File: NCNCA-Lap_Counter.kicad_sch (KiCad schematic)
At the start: 3 parts

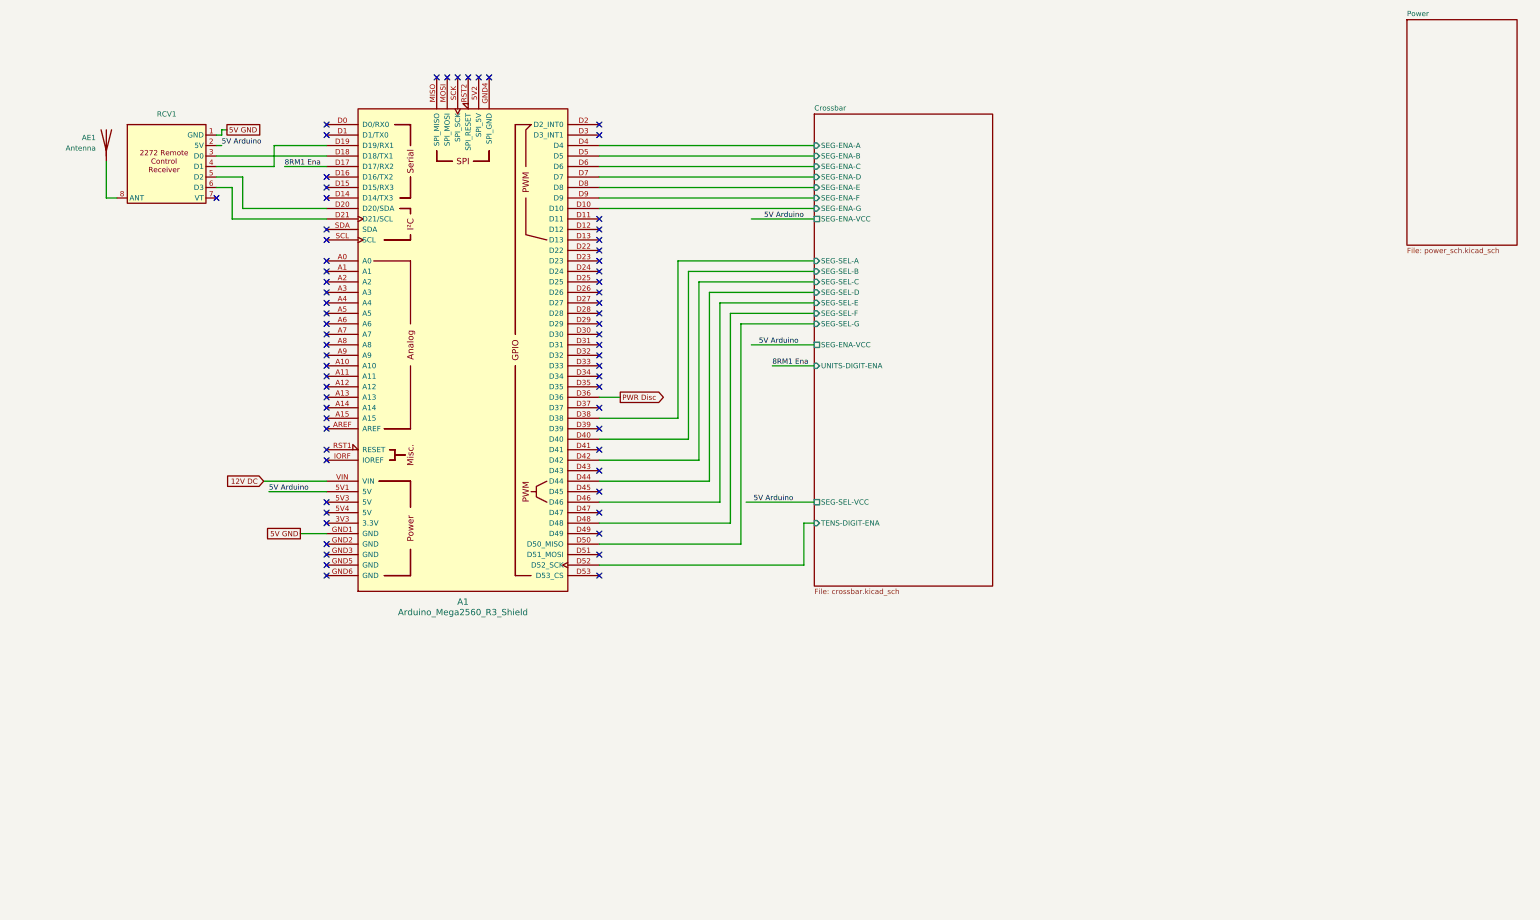
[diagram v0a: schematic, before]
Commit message: Misc clean up
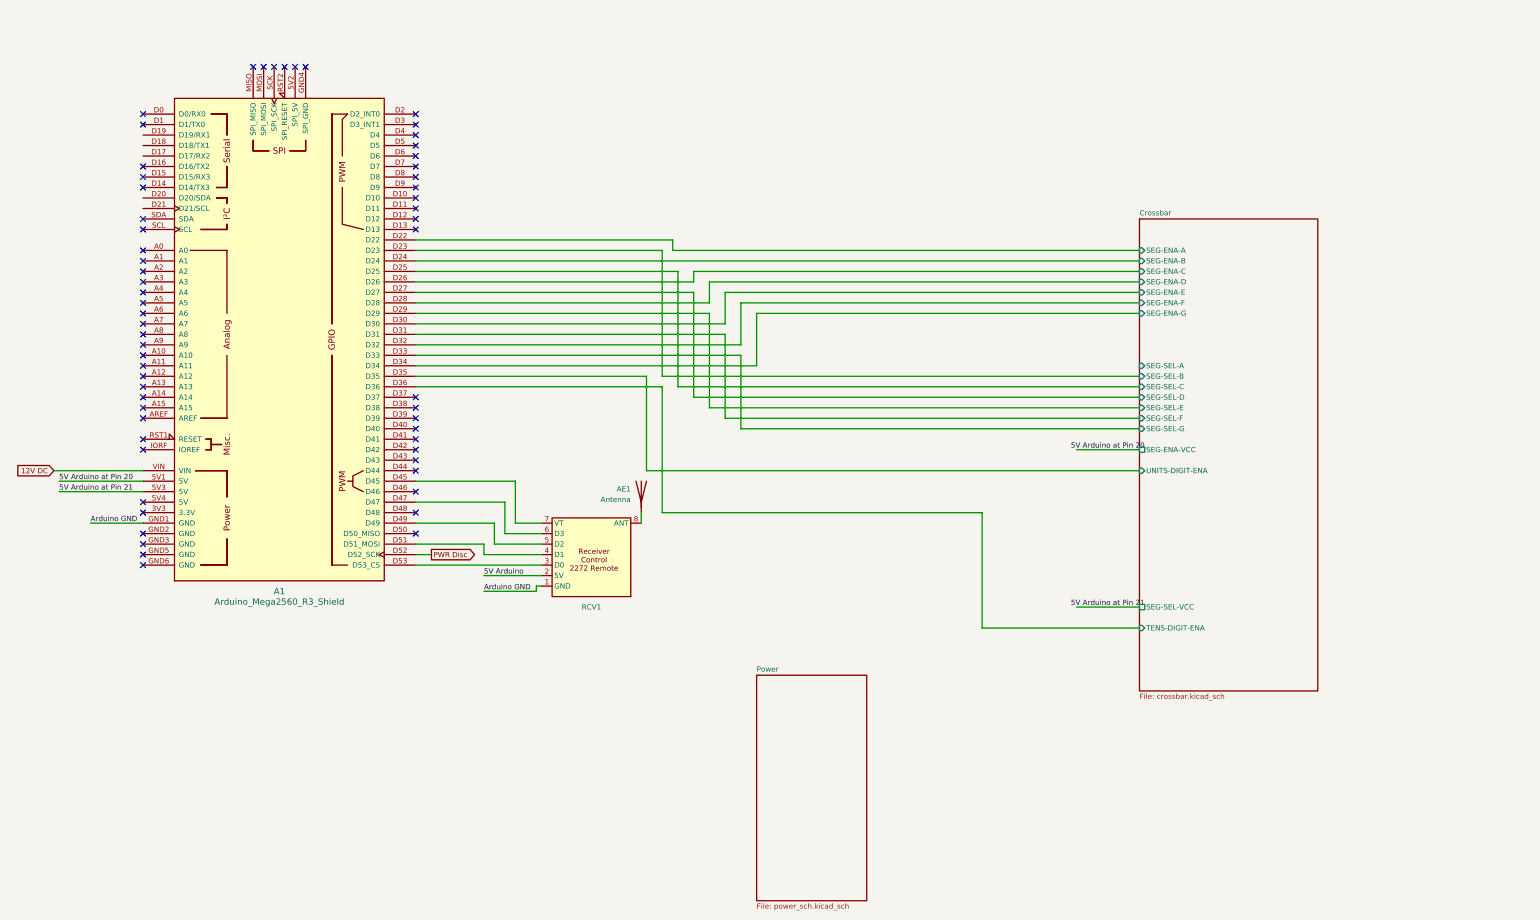
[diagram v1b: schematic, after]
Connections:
- net 5V Arduino: no longer A1.5V1 (5V)
- net Crossbar/SEG-ENA-A: now also A1.D22; no longer A1.D4
- net Crossbar/SEG-ENA-B: now also A1.D24; no longer A1.D5
- net Crossbar/SEG-ENA-C: now also A1.D26; no longer A1.D6
- net Crossbar/SEG-ENA-D: now also A1.D28; no longer A1.D7
- net Crossbar/SEG-ENA-E: now also A1.D30; no longer A1.D8
- net Crossbar/SEG-ENA-F: now also A1.D32; no longer A1.D9
- net Crossbar/SEG-ENA-G: now also A1.D34; no longer A1.D10
- net Crossbar/SEG-SEL-A: no longer A1.D38
- net Crossbar/SEG-SEL-B: now also A1.D23; no longer A1.D40
- net Crossbar/SEG-SEL-C: now also A1.D25; no longer A1.D42
- net Crossbar/SEG-SEL-D: now also A1.D27; no longer A1.D44
- net Crossbar/SEG-SEL-E: now also A1.D29; no longer A1.D46
- net Crossbar/SEG-SEL-F: now also A1.D31; no longer A1.D48
- net Crossbar/SEG-SEL-G: now also A1.D33; no longer A1.D50 (D50_MISO)
- net Crossbar/TENS-DIGIT-ENA: now also A1.D36; no longer A1.D52 (D52_SCK)
- net PWR Disc: now also A1.D52 (D52_SCK); no longer A1.D36
- net at RCV1.3 (D0): now also A1.D53 (D53_CS); no longer A1.D18 (D18/TX1)
- net at RCV1.4 (D1): now also A1.D51 (D51_MOSI); no longer A1.D19 (D19/RX1)
- net at RCV1.5 (D2): now also A1.D49; no longer A1.D20 (D20/SDA)
- net at RCV1.6 (D3): now also A1.D47; no longer A1.D21 (D21/SCL)
- net at RCV1.7 (VT): now also A1.D45
- net 5V Arduino at Pin 21: now reaches A1.5V3 (5V)
- net Crossbar/UNITS-DIGIT-ENA: now reaches A1.D35
- net 5V GND renamed Arduino GND
- net 8RM1 Ena: no longer names the net of A1.D17 (D17/RX2)
- new net 5V Arduino at Pin 20: A1.5V1 (5V)
- no-connect marks 68 -> 61
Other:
- moved on the sheet: A1, AE1, RCV1

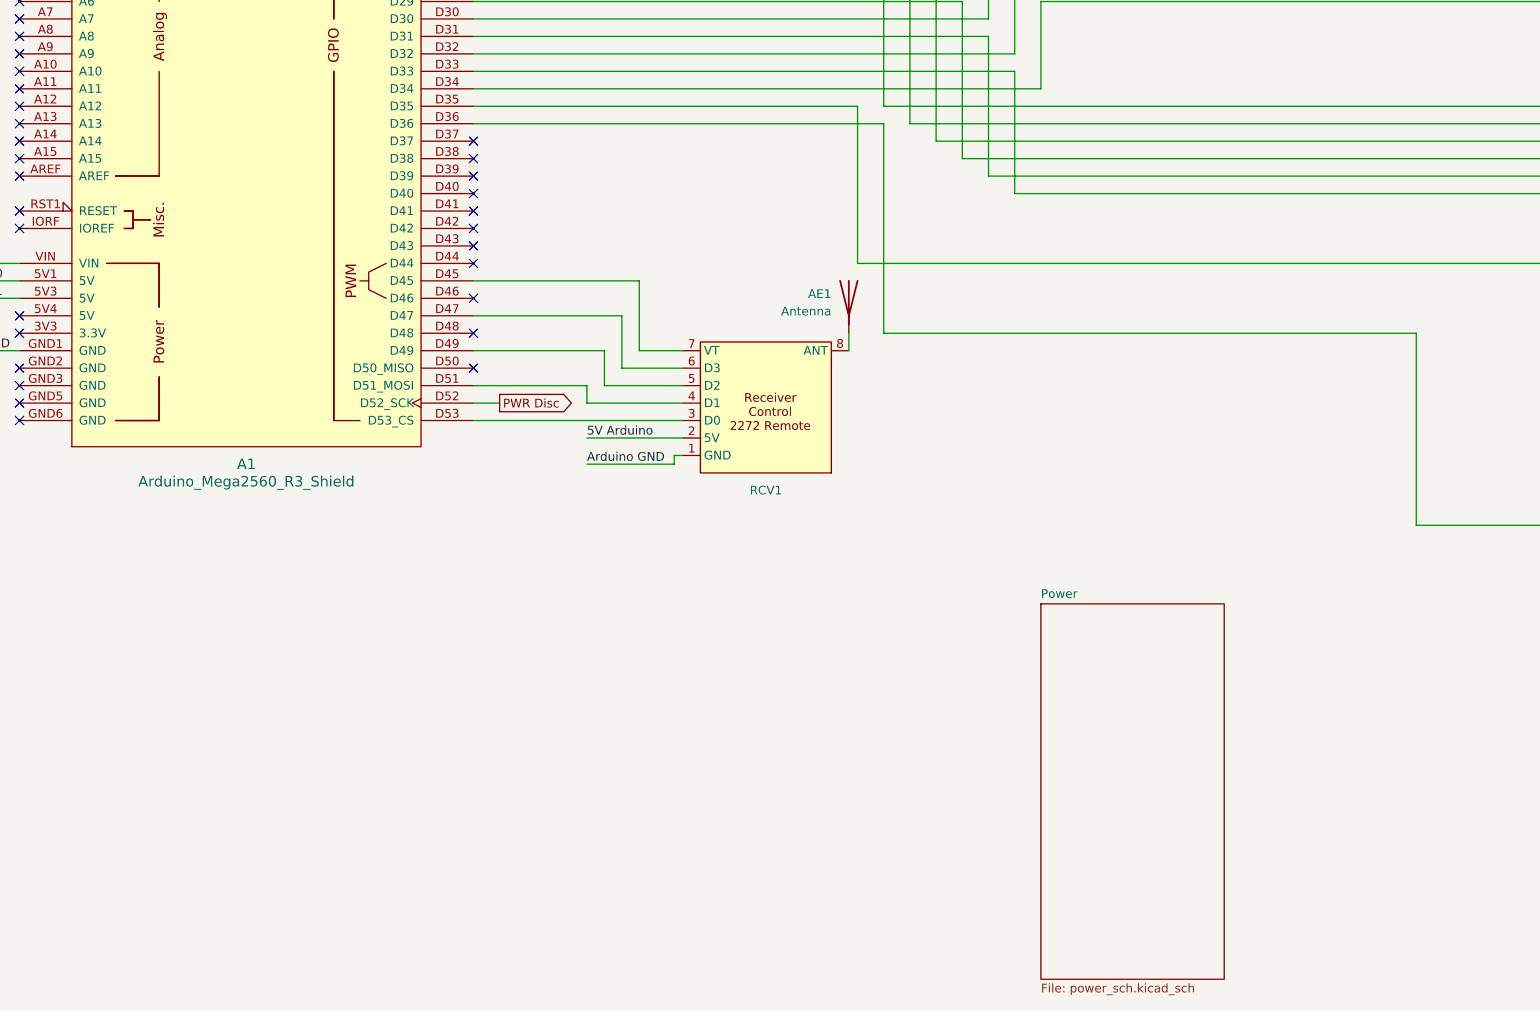
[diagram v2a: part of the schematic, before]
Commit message: Update documen
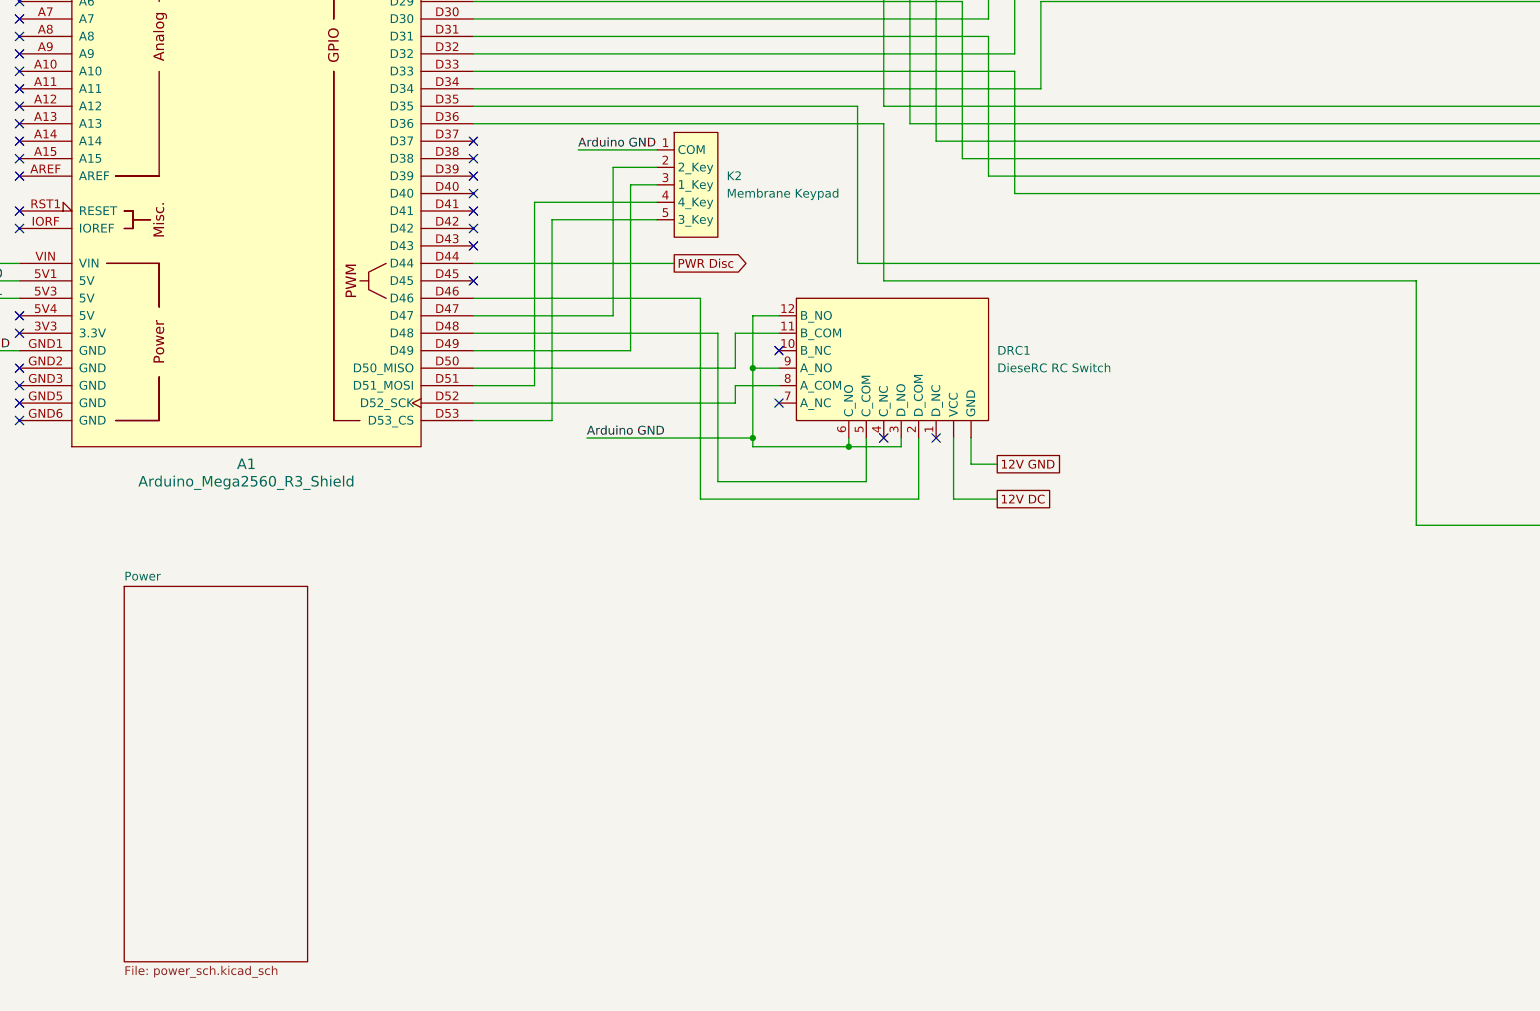
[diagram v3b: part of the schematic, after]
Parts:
- removed AE1: Antenna, symbol Device:Antenna
- removed RCV1: ~, symbol Project Library:Marstech_2272_Receiver
- added DRC1: DieseRC RC Switch, symbol Project Library:DieseRC_Remote_Control_Switch
- added K2: Membrane Keypad, symbol Project Library:Membrane Keypad
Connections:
- net 12V DC: now also DRC1. (VCC)
- net Arduino GND: now also DRC1.12 (B_NO), DRC1.3 (D_NO), DRC1.6 (C_NO), DRC1.9 (A_NO), K2.1 (COM)
- net PWR Disc: now also A1.D44; no longer A1.D52 (D52_SCK)
- net at A1.D53 (D53_CS): now also K2.5 (3_Key)
- net at A1.D51 (D51_MOSI): now also K2.4 (4_Key)
- net at A1.D49: now also K2.3 (1_Key)
- net at A1.D47: now also K2.2 (2_Key)
- net at A1.D46: now also DRC1.2 (D_COM)
- net at A1.D48: now also DRC1.5 (C_COM)
- net at A1.D50 (D50_MISO): now also DRC1.11 (B_COM)
- new net: A1.D52 (D52_SCK), DRC1.8 (A_COM)
- new net 12V GND: DRC1. (VCC)
- no-connect marks 61 -> 62
